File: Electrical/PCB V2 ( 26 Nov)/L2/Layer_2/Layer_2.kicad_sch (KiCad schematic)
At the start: 38 parts, among them J1 Conn_01x02, Q1 AON6354, SW1 SW_Push, U1 LM2596ADJ, U12 VNH5019ATR-E, U2 LM2596ADJ, U3 XT30UPB-M, U4 XT30UPB-M, U5 ESP32-S3-DEVKITM-1-N8

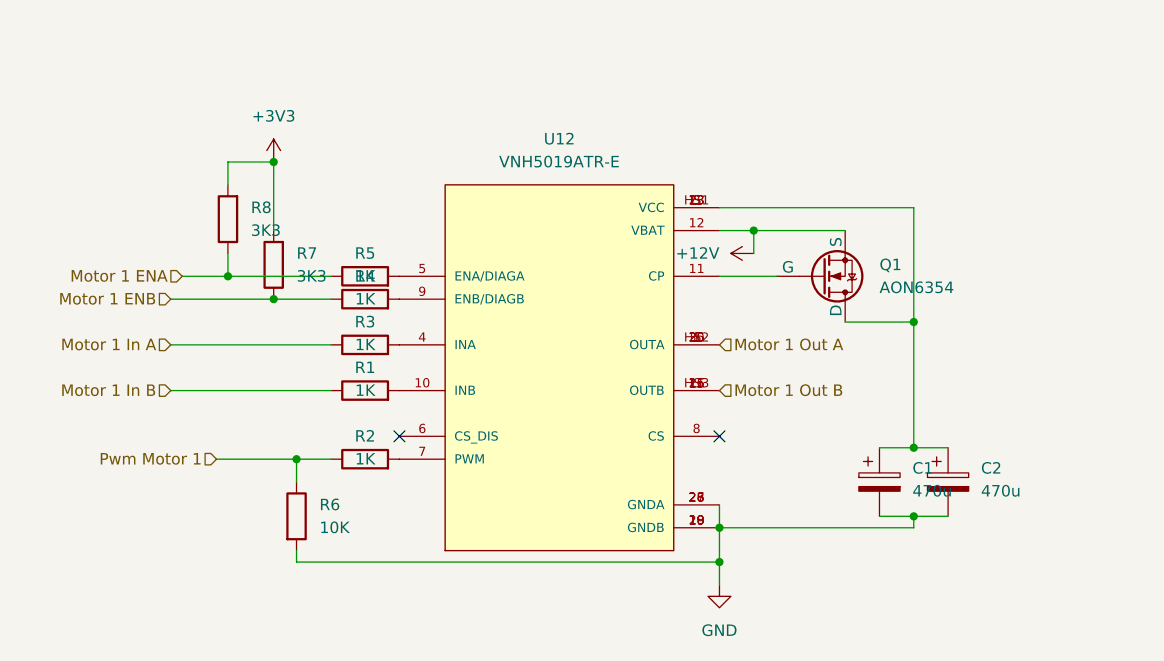
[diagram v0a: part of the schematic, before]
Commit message: updated motor 1 controller cos cx
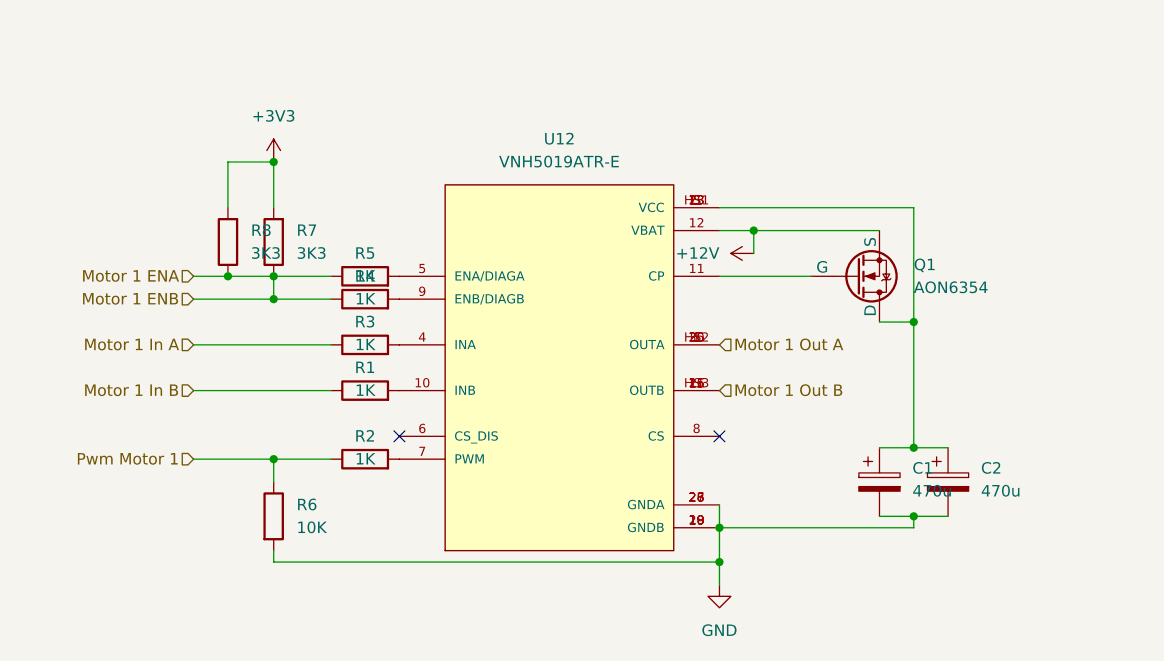
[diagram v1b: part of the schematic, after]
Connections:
- net Motor 1 ENB is gone; now on net Motor 1 ENA: R4.1, R7.1
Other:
- moved on the sheet: Q1, R6, R7, R8
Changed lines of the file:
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@@
 	)
 	(junction
-		(at 39.37 157.48)
+		(at 107.95 142.24)
 		(diameter 0)
 		(color 0 0 0 0)
 	)
 	(junction
-		(at 107.95 142.24)
+		(at 36.83 137.16)
 		(diameter 0)
 		(color 0 0 0 0)
@@
 	)
 	(junction
+		(at 36.83 157.48)
+		(diameter 0)
+		(color 0 0 0 0)
+	)
+	(junction
 		(at 107.95 156.21)
 		(diameter 0)
@@
 	(wire
 		(pts
-			(xy 31.75 134.62) (xy 31.75 137.16)
-		)
-		(stroke
-			(width 0)
-			(type default)
-		)
-	)
-	(wire
-		(pts
 			(xy 104.14 156.21) (xy 107.95 156.21)
 		)
@@
 	(wire
 		(pts
-			(xy 86.36 137.16) (xy 92.71 137.16)
+			(xy 86.36 137.16) (xy 96.52 137.16)
 		)
 		(stroke
@@
 	(wire
 		(pts
-			(xy 39.37 157.48) (xy 30.48 157.48)
+			(xy 107.95 156.21) (xy 111.76 156.21)
 		)
 		(stroke
@@
 	(wire
 		(pts
-			(xy 107.95 156.21) (xy 111.76 156.21)
+			(xy 36.83 168.91) (xy 86.36 168.91)
 		)
 		(stroke
@@
 	(wire
 		(pts
-			(xy 39.37 168.91) (xy 86.36 168.91)
+			(xy 36.83 157.48) (xy 27.94 157.48)
 		)
 		(stroke
@@
 	(wire
 		(pts
-			(xy 31.75 124.46) (xy 31.75 127)
+			(xy 31.75 124.46) (xy 31.75 129.54)
 		)
 		(stroke
@@
 	(wire
 		(pts
-			(xy 31.75 137.16) (xy 43.18 137.16)
+			(xy 31.75 137.16) (xy 36.83 137.16)
 		)
 		(stroke
@@
 	(wire
 		(pts
+			(xy 36.83 137.16) (xy 43.18 137.16)
+		)
+		(stroke
+			(width 0)
+			(type default)
+		)
+	)
+	(wire
+		(pts
+			(xy 36.83 157.48) (xy 43.18 157.48)
+		)
+		(stroke
+			(width 0)
+			(type default)
+		)
+	)
+	(wire
+		(pts
 			(xy 86.36 168.91) (xy 86.36 165.1)
 		)
@@
 	(wire
 		(pts
-			(xy 39.37 157.48) (xy 39.37 160.02)
+			(xy 36.83 157.48) (xy 36.83 160.02)
 		)
 		(stroke
@@
 	(wire
 		(pts
-			(xy 25.4 139.7) (xy 36.83 139.7)
+			(xy 27.94 139.7) (xy 36.83 139.7)
 		)
 		(stroke
@@
 	(wire
 		(pts
-			(xy 39.37 168.91) (xy 39.37 167.64)
+			(xy 36.83 168.91) (xy 36.83 167.64)
 		)
 		(stroke
@@
 	(wire
 		(pts
-			(xy 90.17 132.08) (xy 100.33 132.08)
+			(xy 90.17 132.08) (xy 104.14 132.08)
 		)
 		(stroke
@@
 	(wire
 		(pts
-			(xy 39.37 157.48) (xy 43.18 157.48)
+			(xy 27.94 149.86) (xy 43.18 149.86)
 		)
 		(stroke
@@
 	(wire
 		(pts
-			(xy 26.67 137.16) (xy 31.75 137.16)
+			(xy 16.51 48.26) (xy 29.21 48.26)
 		)
 		(stroke
@@
 	(wire
 		(pts
-			(xy 25.4 149.86) (xy 43.18 149.86)
+			(xy 27.94 137.16) (xy 31.75 137.16)
 		)
 		(stroke
@@
 	(wire
 		(pts
-			(xy 16.51 48.26) (xy 29.21 48.26)
+			(xy 36.83 124.46) (xy 36.83 129.54)
 		)
 		(stroke
@@
 	(wire
 		(pts
-			(xy 36.83 124.46) (xy 36.83 132.08)
+			(xy 104.14 142.24) (xy 107.95 142.24)
 		)
 		(stroke
@@
 	(wire
 		(pts
-			(xy 100.33 142.24) (xy 107.95 142.24)
+			(xy 27.94 144.78) (xy 43.18 144.78)
 		)
 		(stroke
@@
 	(wire
 		(pts
-			(xy 25.4 144.78) (xy 43.18 144.78)
+			(xy 107.95 129.54) (xy 107.95 142.24)
 		)
 		(stroke
@@
 	(wire
 		(pts
-			(xy 107.95 129.54) (xy 107.95 142.24)
+			(xy 31.75 124.46) (xy 36.83 124.46)
 		)
 		(stroke
@@
 	(wire
 		(pts
-			(xy 31.75 124.46) (xy 36.83 124.46)
+			(xy 107.95 163.83) (xy 107.95 165.1)
 		)
 		(stroke
@@
 	(wire
 		(pts
-			(xy 107.95 163.83) (xy 107.95 165.1)
+			(xy 36.83 137.16) (xy 36.83 139.7)
 		)
 		(stroke
@@
 	(hierarchical_label "Pwm Motor 1"
 		(shape input)
-		(at 30.48 157.48 180)
+		(at 27.94 157.48 180)
 		(fields_autoplaced yes)
 		(effects
@@
 	(hierarchical_label "Motor 1 ENA"
 		(shape input)
-		(at 26.67 137.16 180)
+		(at 27.94 137.16 180)
 		(fields_autoplaced yes)
 		(effects
@@
 	(hierarchical_label "Motor 1 In B"
 		(shape input)
-		(at 25.4 149.86 180)
+		(at 27.94 149.86 180)
 		(fields_autoplaced yes)
 		(effects
@@
 	(hierarchical_label "Motor 1 In A"
 		(shape input)
-		(at 25.4 144.78 180)
+		(at 27.94 144.78 180)
 		(fields_autoplaced yes)
 		(effects
@@
 	(hierarchical_label "Motor 1 ENB"
 		(shape input)
-		(at 25.4 139.7 180)
+		(at 27.94 139.7 180)
 		(fields_autoplaced yes)
 		(effects
@@
 	(symbol
 		(lib_id "Device:R")
-		(at 36.83 135.89 180)
+		(at 36.83 133.35 180)
 		(unit 1)
 		(exclude_from_sim no)
@@
 		(dnp no)
 		(property "Reference" "R7"
-			(at 39.37 134.62 0)
+			(at 39.37 132.08 0)
 			(effects
 				(font
@@
 		)
 		(property "Value" "3K3"
-			(at 39.37 137.16 0)
+			(at 39.37 134.62 0)
 			(effects
 				(font
@@
 		)
 		(property "Footprint" "2024l2:res0603"
-			(at 38.608 135.89 90)
+			(at 38.608 133.35 90)
 			(effects
 				(font
@@
 		)
 		(property "Datasheet" "~"
-			(at 36.83 135.89 0)
+			(at 36.83 133.35 0)
 			(effects
 				(font
@@
 		)
 		(property "Description" ""
-			(at 36.83 135.89 0)
+			(at 36.83 133.35 0)
 			(effects
 				(font
@@
 	(symbol
 		(lib_id "vincent:AON6354")
-		(at 92.71 137.16 0)
+		(at 96.52 137.16 0)
 		(mirror x)
 		(unit 1)
@@
 		(fields_autoplaced yes)
 		(property "Reference" "Q1"
-			(at 104.14 135.8899 0)
+			(at 107.95 135.8899 0)
 			(effects
 				(font
@@
 		)
 		(property "Value" "AON6354"
-			(at 104.14 138.4299 0)
+			(at 107.95 138.4299 0)
 			(effects
 				(font
@@
 		)
 		(property "Footprint" "2024l2:8-DFN (5x6)"
-			(at 100.33 134.62 90)
+			(at 104.14 134.62 90)
 			(effects
 				(font
@@
 		)
 		(property "Datasheet" "https://aosmd.com/res/data_sheets/AON6354.pdf"
-			(at 100.33 137.16 0)
+			(at 104.14 137.16 0)
 			(effects
 				(font
@@
 		)
 		(property "Description" ""
-			(at 92.71 137.16 0)
+			(at 96.52 137.16 0)
 			(effects
 				(font
@@
 	(symbol
 		(lib_id "Device:R")
-		(at 39.37 163.83 0)
+		(at 36.83 163.83 0)
 		(unit 1)
 		(exclude_from_sim no)
@@
 		(fields_autoplaced yes)
 		(property "Reference" "R6"
-			(at 41.91 162.5599 0)
+			(at 39.37 162.5599 0)
 			(effects
 				(font
@@
 		)
 		(property "Value" "10K"
-			(at 41.91 165.0999 0)
+			(at 39.37 165.0999 0)
 			(effects
 				(font
@@
 		)
 		(property "Footprint" "2024l2:res0603"
-			(at 37.592 163.83 90)
+			(at 35.052 163.83 90)
 			(effects
 				(font
@@
 		)
 		(property "Datasheet" "~"
-			(at 39.37 163.83 0)
+			(at 36.83 163.83 0)
 			(effects
 				(font
@@
 		)
 		(property "Description" ""
-			(at 39.37 163.83 0)
+			(at 36.83 163.83 0)
 			(effects
 				(font
@@
 	(symbol
 		(lib_id "Device:R")
-		(at 31.75 130.81 180)
+		(at 31.75 133.35 180)
 		(unit 1)
 		(exclude_from_sim no)
@@
 		(dnp no)
 		(property "Reference" "R8"
-			(at 34.29 129.54 0)
+			(at 34.29 132.08 0)
 			(effects
 				(font
@@
 		)
 		(property "Value" "3K3"
-			(at 34.29 132.08 0)
+			(at 34.29 134.62 0)
 			(effects
 				(font
@@
 		)
 		(property "Footprint" "2024l2:res0603"
-			(at 33.528 130.81 90)
+			(at 33.528 133.35 90)
 			(effects
 				(font
@@
 		)
 		(property "Datasheet" "~"
-			(at 31.75 130.81 0)
+			(at 31.75 133.35 0)
 			(effects
 				(font
@@
 		)
 		(property "Description" ""
-			(at 31.75 130.81 0)
+			(at 31.75 133.35 0)
 			(effects
 				(font
